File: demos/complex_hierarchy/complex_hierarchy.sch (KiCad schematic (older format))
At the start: 10 parts, among them P1 CONN_2, P2 CONN_2, U1 ICL7660, U2 78L05

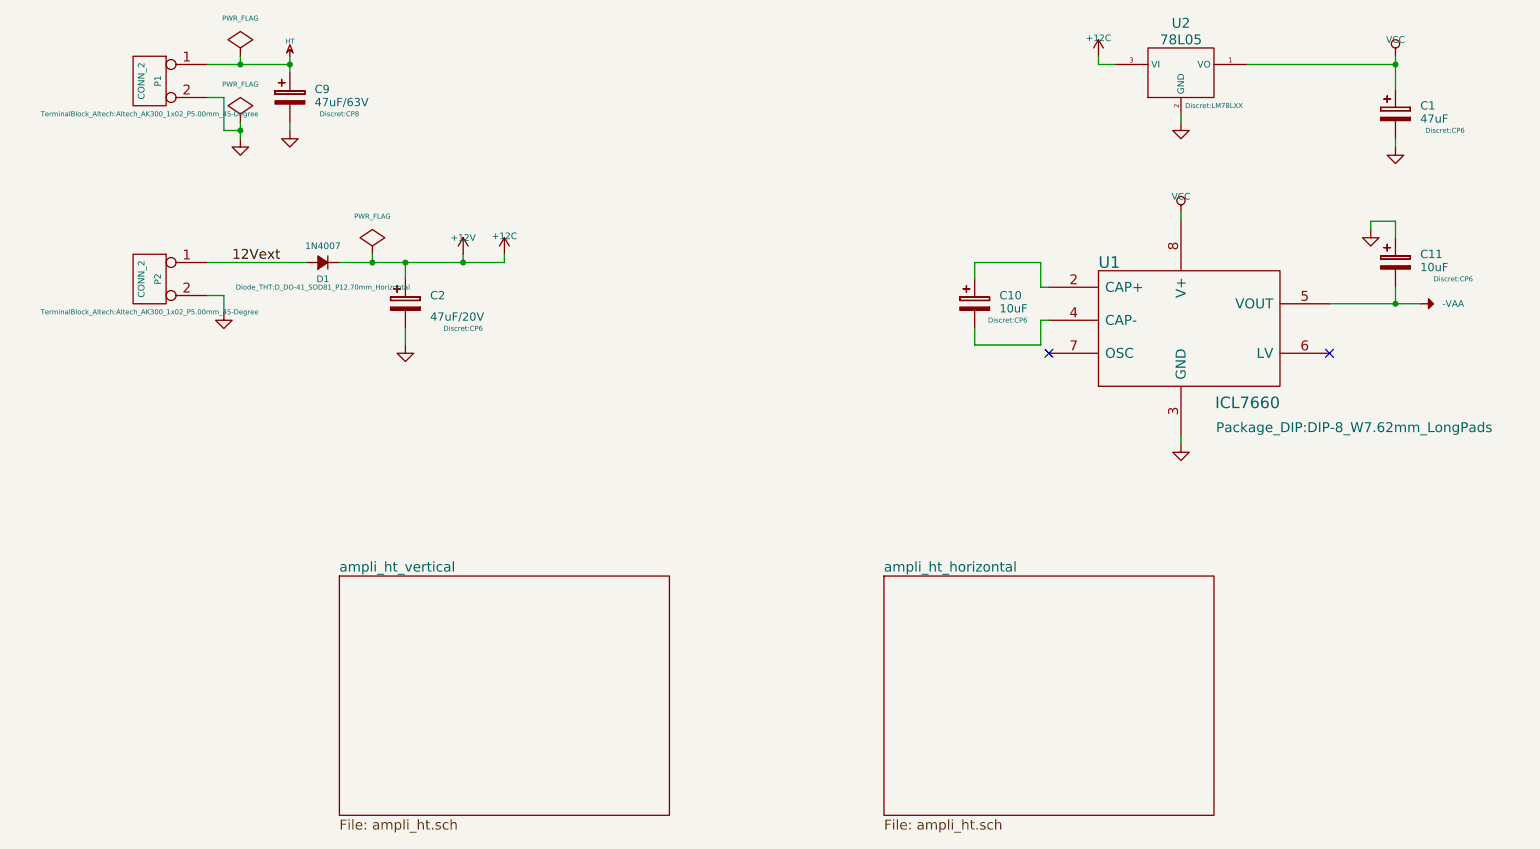
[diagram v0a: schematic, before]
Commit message: Demos update
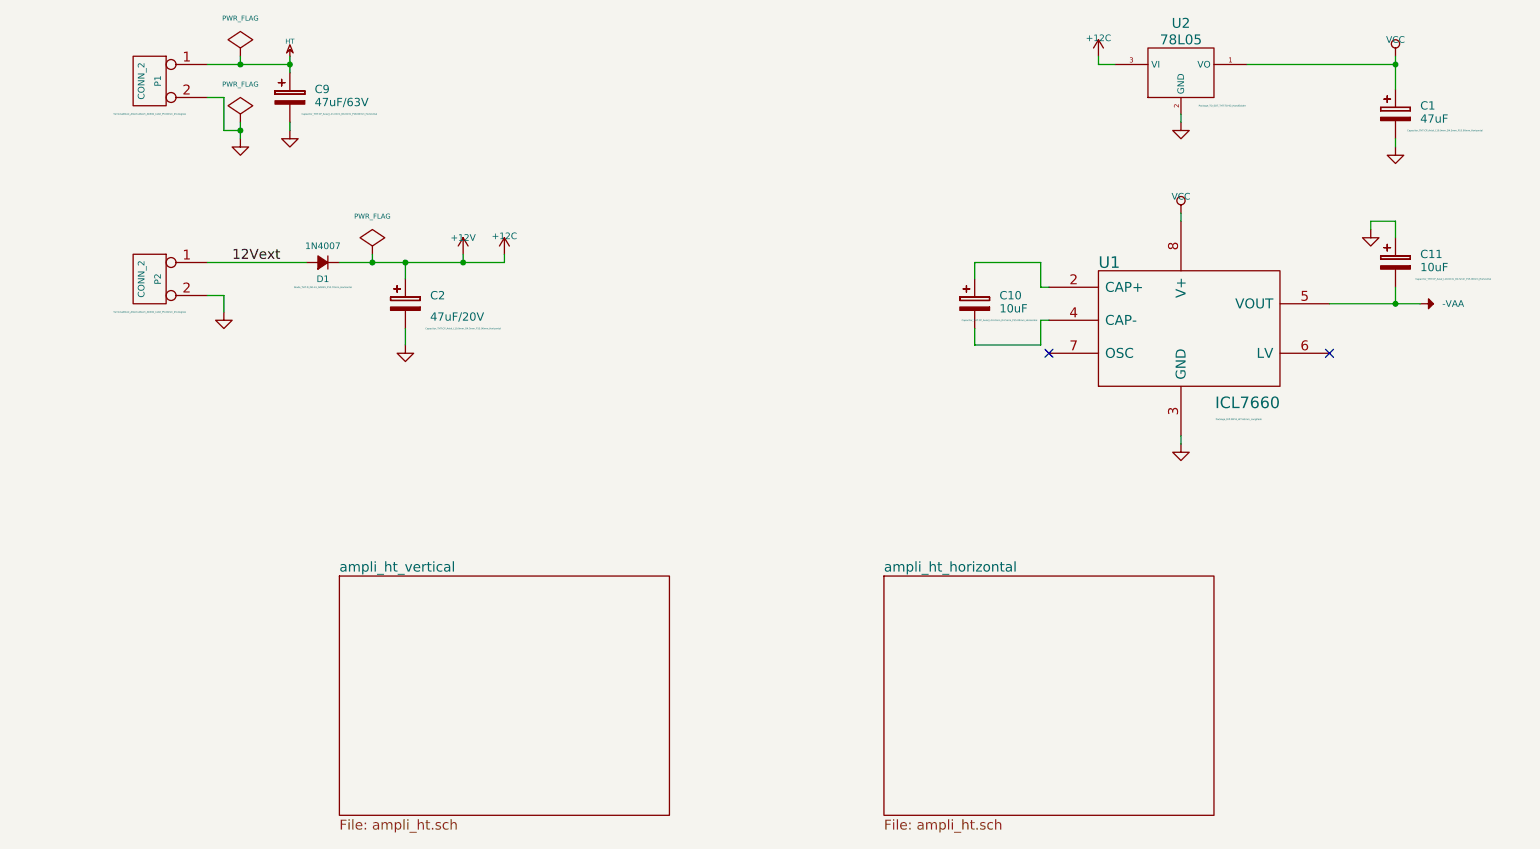
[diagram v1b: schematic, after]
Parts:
- C1, C10, C11, C2: footprint Discret:CP6 -> Capacitor_THT:CP_Axial_L10.0mm_D4.5mm_P15.00mm_Horizontal
- C9: footprint Discret:CP8 -> Capacitor_THT:CP_Axial_L11.0mm_D6.0mm_P18.00mm_Horizontal
- U2: footprint Discret:LM78LXX -> Package_TO_SOT_THT:TO-92_HandSolder
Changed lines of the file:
@@
 EESchema Schematic File Version 5
-LIBS:complex_hierarchy-cache
-EELAYER 29 0
+EELAYER 30 0
 EELAYER END
 $Descr A4 11693 8268
@@
 Comment3 ""
 Comment4 ""
+Comment5 ""
+Comment6 ""
+Comment7 ""
+Comment8 ""
+Comment9 ""
 $EndDescr
 NoConn ~ 8800 3050
@@
 F 0 "C10" H 6800 2800 50  0000 L CNN
 F 1 "10uF" H 6800 2750 50  0000 L TNN
-F 2 "Discret:CP6" H 6850 2650 30  0000 C CNN
+F 2 "Capacitor_THT:CP_Axial_L10.0mm_D4.5mm_P15.00mm_Horizontal" H 6800 2650 10  0000 C CNN
 F 3 "" H 6650 2750 60  0001 C CNN
 	1    6650 2750
@@
 F 0 "#PWR01" H 9050 2300 30  0001 C CNN
 F 1 "GND" H 9050 2230 30  0001 C CNN
-F 2 "" H 9050 2300 60  0001 C CNN
+F 2 "" H 9050 2300 10  0001 C CNN
 F 3 "" H 9050 2300 60  0001 C CNN
 	1    9050 2300
@@
 F 0 "C11" H 9350 2550 50  0000 L CNN
 F 1 "10uF" H 9350 2500 50  0000 L TNN
-F 2 "Discret:CP6" H 9550 2400 30  0000 C CNN
+F 2 "Capacitor_THT:CP_Axial_L10.0mm_D4.5mm_P15.00mm_Horizontal" H 9550 2400 10  0000 C CNN
 F 3 "" H 9200 2500 60  0001 C CNN
 	1    9200 2500
@@
 F 0 "#PWR02" H 9350 2850 20  0001 C CNN
 F 1 "-VAA" V 9350 2950 40  0000 C CNN
-F 2 "" H 9350 2750 60  0001 C CNN
+F 2 "" H 9350 2750 10  0001 C CNN
 F 3 "" H 9350 2750 60  0001 C CNN
 	1    9350 2750
@@
 F 0 "U2" H 7900 1650 60  0000 C CNN
 F 1 "78L05" H 7900 1550 60  0000 C CNN
-F 2 "Discret:LM78LXX" H 8100 1150 30  0000 C CNN
+F 2 "Package_TO_SOT_THT:TO-92_HandSolder" H 8150 1150 10  0000 C CNN
 F 3 "" H 7900 1350 60  0001 C CNN
 	1    7900 1350
@@
 F 0 "#PWR03" H 7900 2300 30  0001 C CNN
 F 1 "VCC" H 7900 2300 40  0000 C CNN
-F 2 "" H 7900 2200 60  0001 C CNN
+F 2 "" H 7900 2200 10  0001 C CNN
 F 3 "" H 7900 2200 60  0001 C CNN
 	1    7900 2200
@@
 F 0 "#PWR04" H 9200 1350 30  0001 C CNN
 F 1 "VCC" H 9200 1350 40  0000 C CNN
-F 2 "" H 9200 1250 60  0001 C CNN
+F 2 "" H 9200 1250 10  0001 C CNN
 F 3 "" H 9200 1250 60  0001 C CNN
 	1    9200 1250
@@
 F 0 "#PWR05" H 7900 3600 30  0001 C CNN
 F 1 "GND" H 7900 3530 30  0001 C CNN
-F 2 "" H 7900 3600 60  0001 C CNN
+F 2 "" H 7900 3600 10  0001 C CNN
 F 3 "" H 7900 3600 60  0001 C CNN
 	1    7900 3600
@@
 F 0 "U1" H 7400 3300 70  0000 L CNN
 F 1 "ICL7660" H 8500 2450 70  0000 R CNN
-F 2 "Package_DIP:DIP-8_W7.62mm_LongPads" H 8950 2300 60  0000 C CNN
+F 2 "Package_DIP:DIP-8_W7.62mm_LongPads" H 8250 2350 10  0000 C CNN
 F 3 "" H 7950 2900 60  0001 C CNN
 	1    7950 2900
@@
 F 0 "C9" H 2650 1550 50  0000 L CNN
 F 1 "47uF/63V" H 2650 1500 50  0000 L TNN
-F 2 "Discret:CP8" H 2800 1400 30  0000 C CNN
+F 2 "Capacitor_THT:CP_Axial_L11.0mm_D6.0mm_P18.00mm_Horizontal" H 2800 1400 10  0000 C CNN
 F 3 "" H 2500 1500 60  0001 C CNN
 	1    2500 1500
@@
 F 0 "#PWR06" H 2500 1700 30  0001 C CNN
 F 1 "GND" H 2500 1630 30  0001 C CNN
-F 2 "" H 2500 1700 60  0001 C CNN
+F 2 "" H 2500 1700 10  0001 C CNN
 F 3 "" H 2500 1700 60  0001 C CNN
 	1    2500 1700
@@
 F 0 "#PWR07" H 2200 1750 30  0001 C CNN
 F 1 "GND" H 2200 1680 30  0001 C CNN
-F 2 "" H 2200 1750 60  0001 C CNN
+F 2 "" H 2200 1750 10  0001 C CNN
 F 3 "" H 2200 1750 60  0001 C CNN
 	1    2200 1750
@@
 F 0 "P1" V 1600 1400 40  0000 C CNN
 F 1 "CONN_2" V 1700 1400 40  0000 C CNN
-F 2 "TerminalBlock_Altech:Altech_AK300_1x02_P5.00mm_45-Degree" H 1650 1200 30  0000 C CNN
+F 2 "TerminalBlock_Altech:Altech_AK300_1x02_P5.00mm_45-Degree" H 1650 1200 10  0000 C CNN
 F 3 "" H 1650 1400 60  0001 C CNN
 	1    1650 1400
@@
 F 0 "#PWR08" H 2500 1370 20  0001 C CNN
 F 1 "HT" H 2500 1340 30  0000 C CNN
-F 2 "" H 2500 1250 60  0001 C CNN
+F 2 "" H 2500 1250 10  0001 C CNN
 F 3 "" H 2500 1250 60  0001 C CNN
 	1    2500 1250
@@
 F 0 "C1" H 9350 1650 50  0000 L CNN
 F 1 "47uF" H 9350 1600 50  0000 L TNN
-F 2 "Discret:CP6" H 9500 1500 30  0000 C CNN
+F 2 "Capacitor_THT:CP_Axial_L10.0mm_D4.5mm_P15.00mm_Horizontal" H 9500 1500 10  0000 C CNN
 F 3 "" H 9200 1600 60  0001 C CNN
 	1    9200 1600
@@
 F 0 "#PWR09" H 9200 1800 30  0001 C CNN
 F 1 "GND" H 9200 1730 30  0001 C CNN
-F 2 "" H 9200 1800 60  0001 C CNN
+F 2 "" H 9200 1800 10  0001 C CNN
 F 3 "" H 9200 1800 60  0001 C CNN
 	1    9200 1800
@@
 F 0 "#PWR010" H 7900 1650 30  0001 C CNN
 F 1 "GND" H 7900 1580 30  0001 C CNN
-F 2 "" H 7900 1650 60  0001 C CNN
+F 2 "" H 7900 1650 10  0001 C CNN
 F 3 "" H 7900 1650 60  0001 C CNN
 	1    7900 1650
@@
 F 0 "#PWR011" H 7400 1220 30  0001 C CNN
 F 1 "+12C" H 7400 1360 40  0000 C CNN
-F 2 "" H 7400 1250 60  0001 C CNN
+F 2 "" H 7400 1250 10  0001 C CNN
 F 3 "" H 7400 1250 60  0001 C CNN
 	1    7400 1250
@@
 F 0 "#U012" H 2200 1520 30  0001 C CNN
 F 1 "PWR_FLAG" H 2200 1480 30  0000 C CNN
-F 2 "" H 2200 1250 60  0001 C CNN
+F 2 "" H 2200 1250 10  0001 C CNN
 F 3 "" H 2200 1250 60  0001 C CNN
 	1    2200 1250
@@
 F 0 "#U013" H 3000 2720 30  0001 C CNN
 F 1 "PWR_FLAG" H 3000 2680 30  0000 C CNN
-F 2 "" H 3000 2450 60  0001 C CNN
+F 2 "" H 3000 2450 10  0001 C CNN
 F 3 "" H 3000 2450 60  0001 C CNN
 	1    3000 2450
@@
 F 0 "#PWR014" H 3800 2420 30  0001 C CNN
 F 1 "+12C" H 3800 2560 40  0000 C CNN
-F 2 "" H 3800 2450 60  0001 C CNN
+F 2 "" H 3800 2450 10  0001 C CNN
 F 3 "" H 3800 2450 60  0001 C CNN
 	1    3800 2450
@@
 F 0 "#U015" H 2200 1920 30  0001 C CNN
 F 1 "PWR_FLAG" H 2200 1880 30  0000 C CNN
-F 2 "" H 2200 1650 60  0001 C CNN
+F 2 "" H 2200 1650 10  0001 C CNN
 F 3 "" H 2200 1650 60  0001 C CNN
 	1    2200 1650
@@
 F 0 "#U016" H 3550 2400 20  0001 C CNN
 F 1 "+12V" H 3550 2550 40  0000 C CNN
-F 2 "" H 3550 2450 60  0001 C CNN
+F 2 "" H 3550 2450 10  0001 C CNN
 F 3 "" H 3550 2450 60  0001 C CNN
 	1    3550 2450
@@
 F 0 "#PWR017" H 3200 3000 30  0001 C CNN
 F 1 "GND" H 3200 2930 30  0001 C CNN
-F 2 "" H 3200 3000 60  0001 C CNN
+F 2 "" H 3200 3000 10  0001 C CNN
 F 3 "" H 3200 3000 60  0001 C CNN
 	1    3200 3000
@@
 F 0 "C2" H 3350 2800 50  0000 L CNN
 F 1 "47uF/20V" H 3350 2700 50  0000 L TNN
-F 2 "Discret:CP6" H 3550 2600 30  0000 C CNN
+F 2 "Capacitor_THT:CP_Axial_L10.0mm_D4.5mm_P15.00mm_Horizontal" H 3550 2600 10  0000 C CNN
 F 3 "" H 3200 2750 60  0001 C CNN
 	1    3200 2750
@@
 F 0 "D1" H 2700 2400 40  0000 C CNN
 F 1 "1N4007" H 2700 2600 40  0000 C CNN
-F 2 "Diode_THT:D_DO-41_SOD81_P12.70mm_Horizontal" H 2700 2350 30  0000 C CNN
+F 2 "Diode_THT:D_DO-41_SOD81_P12.70mm_Horizontal" H 2700 2350 10  0000 C CNN
 F 3 "" H 2700 2500 60  0001 C CNN
 	1    2700 2500
@@
 F 0 "#PWR018" H 2100 2800 30  0001 C CNN
 F 1 "GND" H 2100 2730 30  0001 C CNN
-F 2 "" H 2100 2800 60  0001 C CNN
+F 2 "" H 2100 2800 10  0001 C CNN
 F 3 "" H 2100 2800 60  0001 C CNN
 	1    2100 2800
@@
 F 0 "P2" V 1600 2600 40  0000 C CNN
 F 1 "CONN_2" V 1700 2600 40  0000 C CNN
-F 2 "TerminalBlock_Altech:Altech_AK300_1x02_P5.00mm_45-Degree" H 1650 2400 30  0000 C CNN
+F 2 "TerminalBlock_Altech:Altech_AK300_1x02_P5.00mm_45-Degree" H 1650 2400 10  0000 C CNN
 F 3 "" H 1650 2600 60  0001 C CNN
 	1    1650 2600
